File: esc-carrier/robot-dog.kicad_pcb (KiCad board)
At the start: 2 copper layers, 35 parts, among them J1 Conn_01x02, J10 Conn_01x02, J11 Conn_01x04, J12 Conn_01x04, J13 Conn_01x04, J2 Conn_01x04, J3 Conn_01x04, J4 Conn_01x03, J5 Conn_01x05, J6 Conn_01x05, J7 Conn_01x05, J8 Conn_01x02, J9 Conn_01x02, SW1 SW_DIP_x02

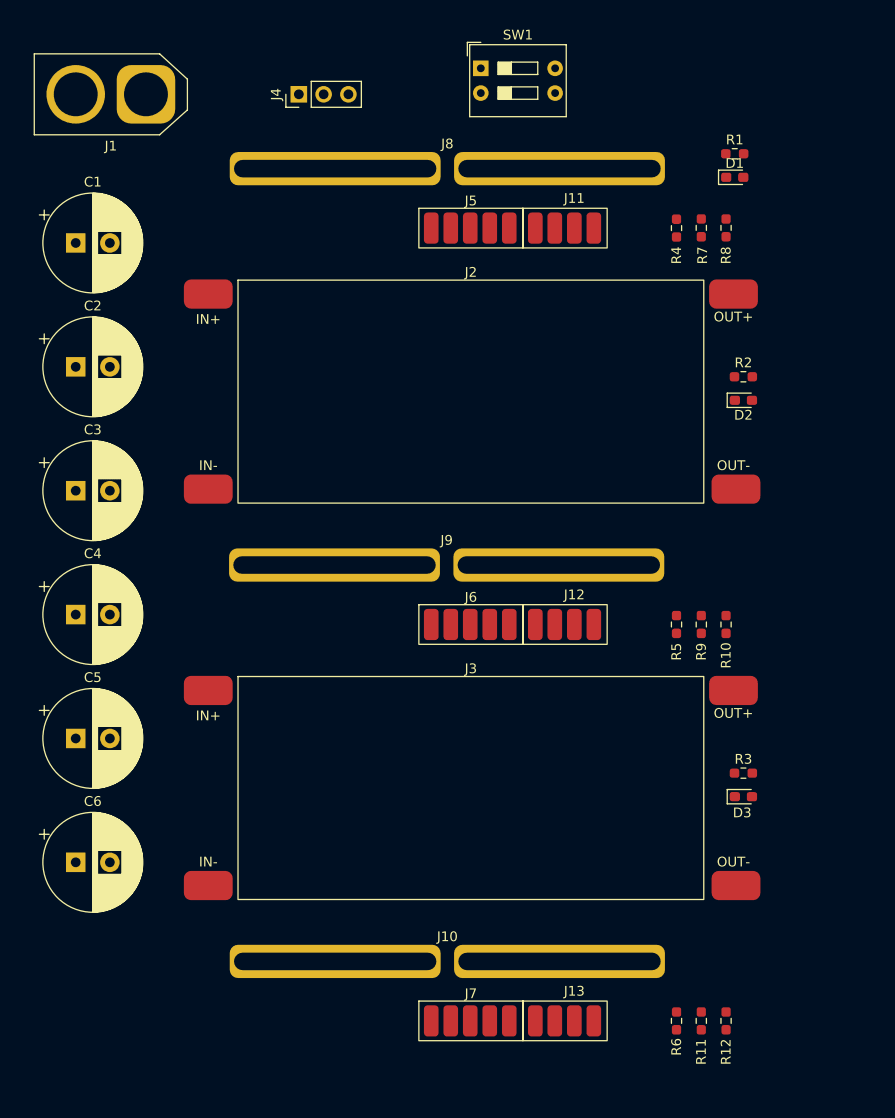
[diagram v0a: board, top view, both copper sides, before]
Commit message: start trace routing
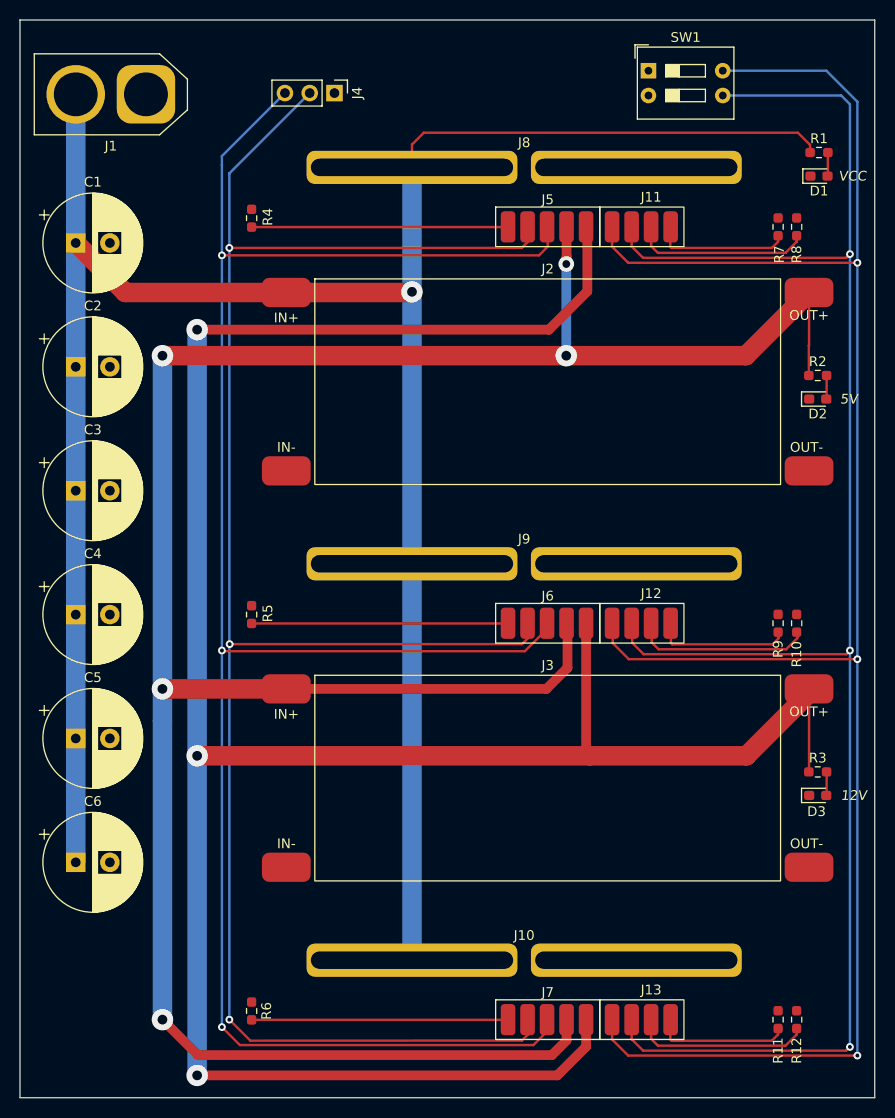
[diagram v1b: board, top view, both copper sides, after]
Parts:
- moved R4 43.6 mm to (155.2, 58.4)
- moved R5 43.6 mm to (155.2, 99.1)
- moved R6 43.6 mm to (155.2, 139.7)
- moved SW1 17.2 mm to (195.9, 43.3)
- moved D1 8.64 mm to (213.4, 54.1)
- moved R1 8.64 mm to (213.4, 51.7)
- moved J3 8.62 mm to (185.5, 115.8)
- moved J2 8.62 mm to (185.5, 75.2)
- moved J9 7.95 mm to (183.1, 93.9)
- moved J13 7.88 mm to (192.2, 140.6)
- moved R11 7.88 mm to (209.2, 140.6)
- moved J11 7.88 mm to (192.2, 59.3)
- moved J12 7.88 mm to (192.2, 99.9)
- moved J10 7.88 mm to (183.1, 134.5)
- moved J7 7.88 mm to (181.5, 140.6)
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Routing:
- net +12V: track 0.00 -> 256.4 mm, vias 0 -> 3
- net +5V: track 0.00 -> 251.6 mm, vias 0 -> 5
- net VCC: track 0.00 -> 241.6 mm, vias 0 -> 1
- net SDA: track 0.00 -> 205.1 mm, vias 0 -> 3
- net SCL: track 0.00 -> 196.6 mm, vias 0 -> 3
- net Net-(J11-Pad1): track 0.00 -> 196.4 mm, vias 0 -> 3
- net Net-(J11-Pad2): track 0.00 -> 185.1 mm, vias 0 -> 3
- net Net-(J7-Pad1): track 0.00 -> 27.3 mm
- net Net-(J6-Pad1): track 0.00 -> 26.3 mm
- net Net-(J5-Pad1): track 0.00 -> 26.3 mm
- net Net-(J13-Pad3): track 0.00 -> 18.9 mm
- net Net-(J12-Pad3): track 0.00 -> 18.3 mm
- net Net-(J11-Pad3): track 0.00 -> 18.3 mm
- net Net-(J12-Pad4): track 0.00 -> 14.0 mm
- net Net-(J11-Pad4): track 0.00 -> 14.0 mm
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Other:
- board outline added: 87.6 x 110.5 mm
- board text added: "12V"
- board text added: "5V"
- board text added: "VCC"
